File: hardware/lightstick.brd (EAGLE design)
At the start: 55 x 35 mm, 14 parts, among them U1 MCP1703AT-3302E/CB, X1 RIA182-02, X2 RIA182-02

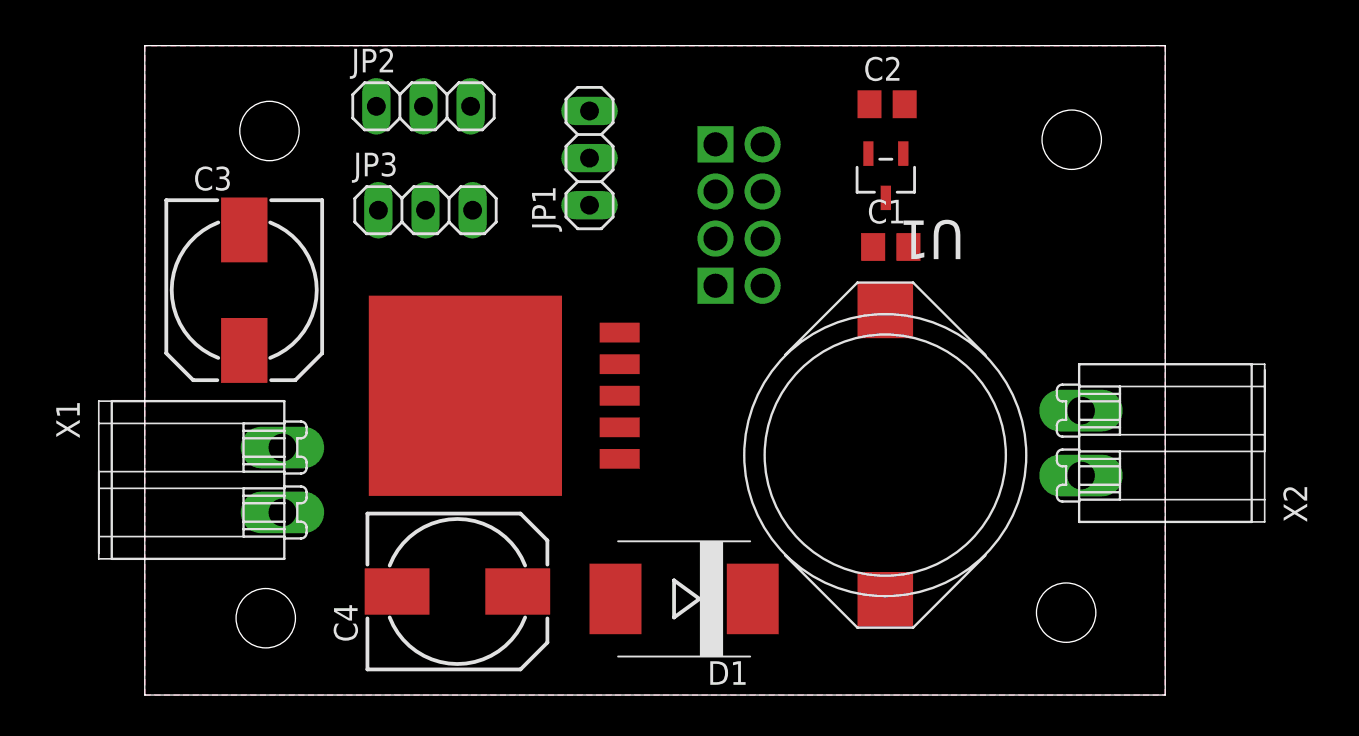
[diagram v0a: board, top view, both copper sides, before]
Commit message: new layout + routing
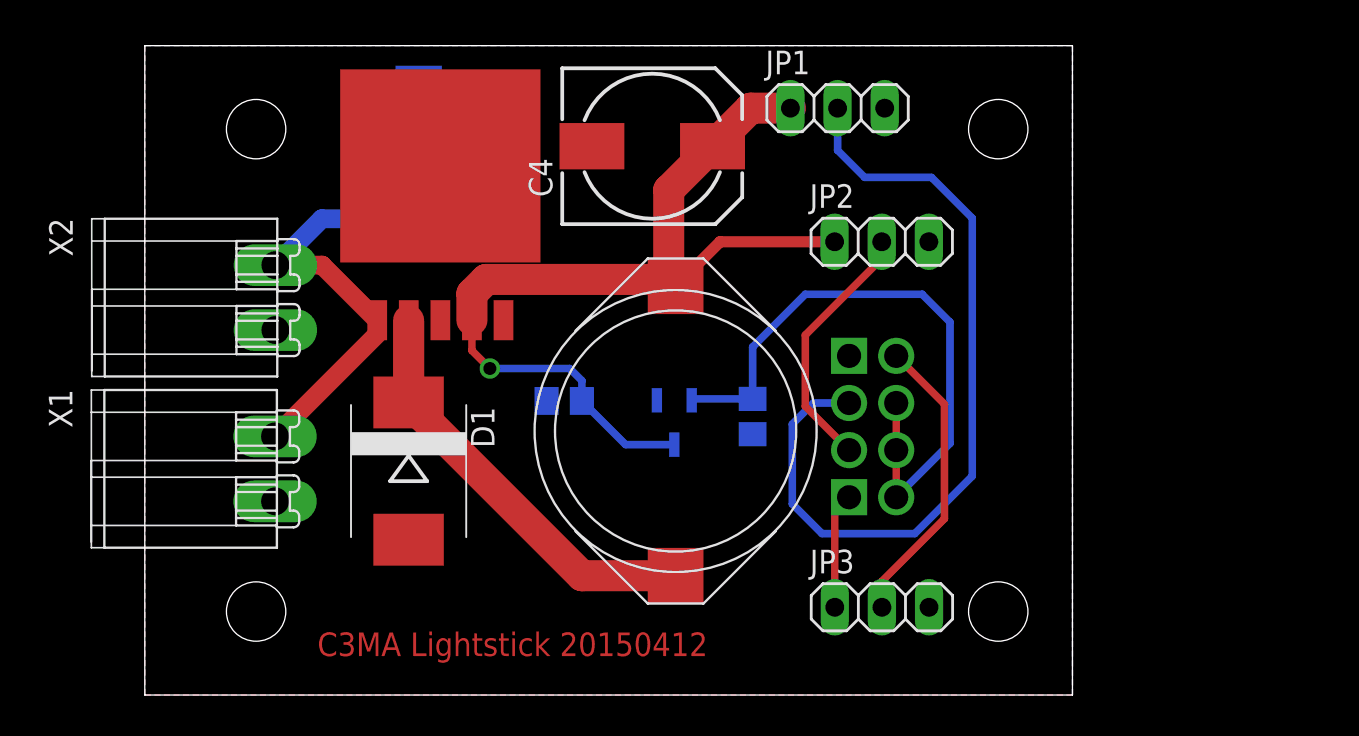
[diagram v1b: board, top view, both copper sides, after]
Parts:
- moved X2 44.9 mm to (7.04, 23.2), turned to 270 degrees
- moved JP3 32.6 mm to (39.7, 4.73)
- moved C4 26.2 mm to (27.4, 29.6)
- moved JP2 25.8 mm to (39.7, 24.4)
- moved C1 19.5 mm to (22.6, 15.8), flipped to the bottom
- moved C2 18.3 mm to (32.8, 15.0), flipped to the bottom, turned to 270 degrees
- moved U1 17.5 mm to (28.5, 14.7), flipped to the bottom
- moved D1 16.4 mm to (14.2, 12.1), turned to 270 degrees
- moved JP1 13.6 mm to (37.3, 31.6), turned to 0 degrees
- moved U$1 13.5 mm to (30.3, 14.5)
- moved U$2 12.5 mm to (15.9, 28.5), turned to 270 degrees
- moved C3 11.8 mm to (14.8, 28.9), flipped to the bottom
- moved L1 11.4 mm to (28.6, 14.2)
- moved X1 0.72 mm to (7.02, 13.9)
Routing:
- net +5V: track 0.00 -> 50.9 mm, vias 0 -> 1
- net DATA: track 0.00 -> 44.4 mm
- net +3V3: track 0.00 -> 34.3 mm
- net +12V: track 0.00 -> 24.0 mm
- net N$1: track 0.00 -> 22.7 mm
- net TX: track 0.00 -> 16.0 mm
- net PROGRAM: track 0.00 -> 13.9 mm
- net RX: track 0.00 -> 6.25 mm
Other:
- board size 55 x 35 mm -> 50 x 35 mm
- board text added: "C3MA Lightstick 20150412"
